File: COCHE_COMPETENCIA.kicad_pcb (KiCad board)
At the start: 2 copper layers, 90 x 65 mm, 25 parts, among them J1 BAT, J2 SENSORES, J3 M1, J4 M2, SW1 SW_Push, SW2 SW_Push, U1 L7805, U2 ESP32-DEVKIT-V1, U3 DRV8833, U4 DRV8833

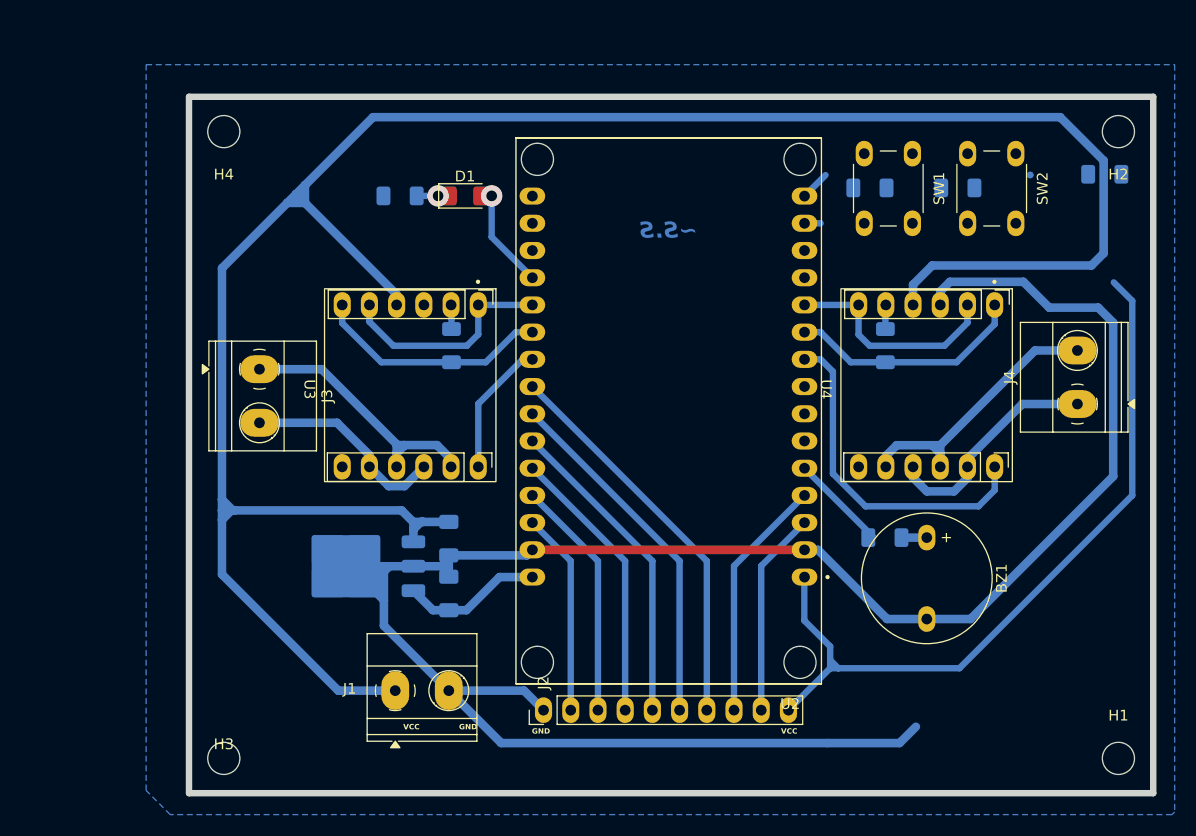
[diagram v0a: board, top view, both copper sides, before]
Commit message: V1 - MotorBoard 2025
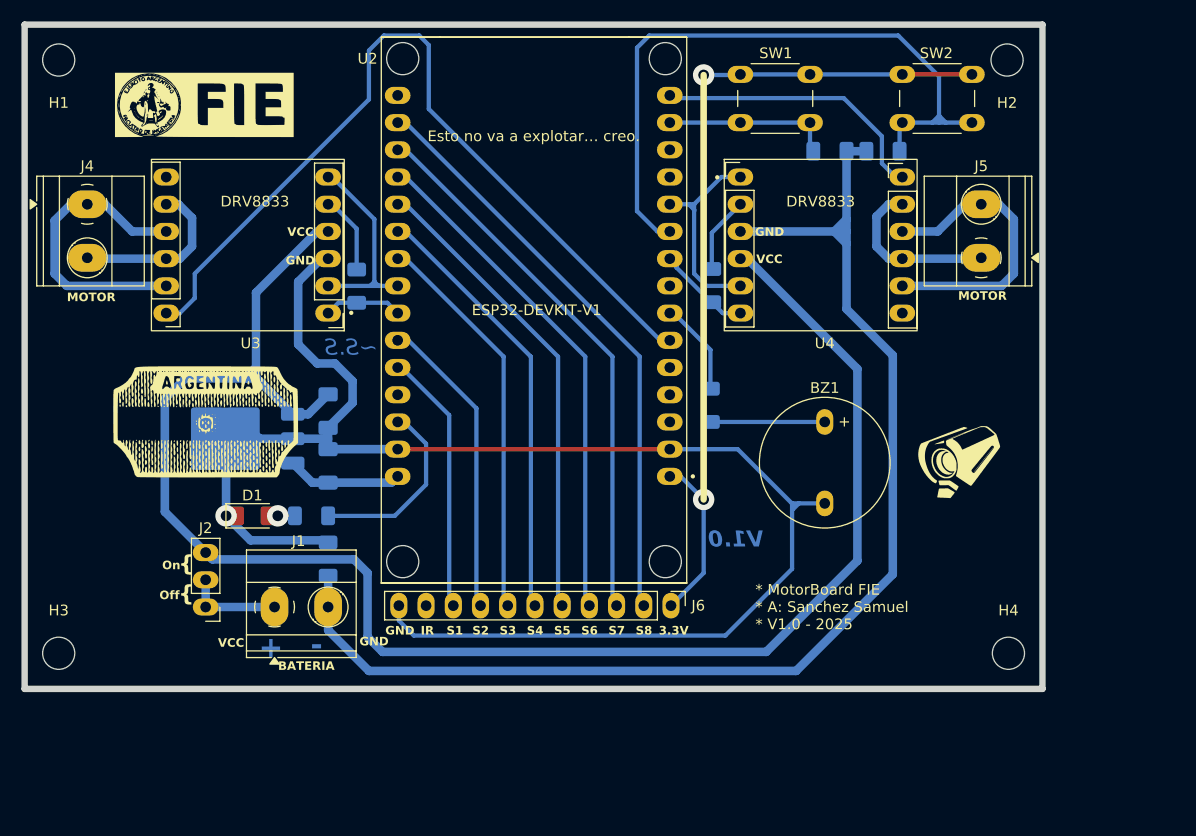
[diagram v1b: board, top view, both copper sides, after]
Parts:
- added G***: LOGO, LOGO, F.Cu at (114.6, 61.8)
- added G***: LOGO, LOGO, F.Cu at (184.8, 65.6)
- added G***: LOGO, LOGO, F.Cu at (114.4, 32.3)
- added J6: SENSORES, Connector_PinHeader_2.54mm:PinHeader_1x11_P2.54mm_Vertical, F.Cu at (158.0, 79.0)
- J2: value SENSORES -> SWITCH; footprint Connector_PinHeader_2.54mm:PinHeader_1x10_P2.54mm_Vertical -> Connector_PinHeader_2.54mm:PinHeader_1x03_P2.54mm_Vertical
- R1: value 10k -> 0
- R3: value 220 -> 10k
- R4: value 0 -> 220
- moved H1 118.5 mm to (100.8, 28.1), turned to 180 degrees
- moved H4 87.9 mm to (189.5, 83.4), turned to 0 degrees
- moved R1 61.3 mm to (126.0, 74.7), turned to -90 degrees
- moved R5 54.6 mm to (128.7, 49.2), turned to 90 degrees
- moved R3 45.3 mm to (177.8, 36.6)
- moved R7 42.7 mm to (161.7, 60.3), turned to -90 degrees
- moved D1 35.9 mm to (118.9, 70.6)
- moved J2 33.0 mm to (114.6, 79.1), turned to 180 degrees
- moved U3 24.0 mm to (118.1, 35.4), turned to 180 degrees
- moved J4 22.3 mm to (103.5, 41.5)
- moved R4 20.6 mm to (124.4, 70.6), turned to 180 degrees
- moved H3 18.3 mm to (100.8, 83.4)
- moved SW1 17.7 mm to (164.5, 29.4), turned to 0 degrees
- moved R6 17.1 mm to (161.8, 49.1)
- moved C1 16.4 mm to (126.0, 60.8)
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- renumbered J3 to J4, J4 to J5
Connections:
- net Net-(U1-OUT) renamed +5V
- D1 pad 1: Net-(D1-K) -> GND
- D1 pad 2: /LED_LARGADA -> Net-(D1-A)
- J1 pad 1: VCC -> Net-(J1-Pin_1)
- J2 pad 1: GND -> Net-(J1-Pin_1)
- J2 pad 2: /S1 -> Net-(J1-Pin_1)
- J2 pad 3: /S2 -> VCC
- R1 pad 1: /SW1 -> GND
- R2 pad 1: /SW2 -> /SW1
- R3 pad 1: Net-(D1-K) -> /SW2
- R4 pad 1: /IN_M1_B -> /LED_LARGADA
- R4 pad 2: Net-(U3-IN3) -> Net-(D1-A)
- R5 pad 1: /BUZZER -> /IN_M1_A
- R5 pad 2: Net-(BZ1-+) -> Net-(U3-IN2)
- R6 pad 1: /IN_M2_A -> /IN_M2_B
- R6 pad 2: Net-(U4-IN2) -> Net-(U4-IN3)
- R7 pad 1: +3.3V -> /BUZZER
- R7 pad 2: Net-(R7-Pad2) -> Net-(BZ1-+)
- SW1 pad 1: Net-(R7-Pad2) -> +3.3V
- SW2 pad 1: Net-(R7-Pad2) -> +3.3V
- U2 pad 10: /IN_M2_A -> /SW2
- U2 pad 11: /IN_M2_B -> /IN_M2_A
- U2 pad 14: /SW2 -> /SW1
- U2 pad 15: /SW1 -> /SLEEP_M2
- U2 pad 17: unconnected-(U2-VP-Pad17) -> /S8
- U2 pad 18: unconnected-(U2-VN-Pad18) -> /S7
- U2 pad 19: /LED_LARGADA -> /S6
- U2 pad 20: /IN_M1_A -> /S5
- U2 pad 21: /IN_M1_B -> /S4
- U2 pad 22: /SLEEP_M1 -> /S3
- U2 pad 23: /S6 -> /IN_M1_B
- U2 pad 24: /S5 -> /IN_M1_A
- U2 pad 25: /S4 -> /S2
- U2 pad 26: /S3 -> /S1
- U2 pad 27: /S2 -> unconnected-(U2-D12-Pad27)
- U2 pad 28: /S1 -> /LED_LARGADA
- U2 pad 3: /S8 -> unconnected-(U2-D15-Pad3)
- U2 pad 4: /S7 -> unconnected-(U2-D2-Pad4)
- U2 pad 5: /BUZZER -> unconnected-(U2-D4-Pad5)
- U2 pad 6: unconnected-(U2-RX2-Pad6) -> /SLEEP_M1
- U2 pad 7: unconnected-(U2-TX2-Pad7) -> /BUZZER
- U2 pad 9: /SLEEP_M2 -> /IN_M2_B
- U3 pad 2: Net-(U3-IN3) -> /IN_M1_B
- U3 pad 5: /IN_M1_A -> Net-(U3-IN2)
- U4 pad 2: /IN_M2_B -> Net-(U4-IN3)
- U4 pad 5: Net-(U4-IN2) -> /IN_M2_A
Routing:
- net GND: track 188.5 -> 269.8 mm, vias 0 -> 1
- net /SLEEP_M1: track 12.7 -> 77.0 mm
- net /SW2: track 1.56 -> 64.7 mm
- net VCC: track 213.9 -> 157.4 mm
- net /S8: track 19.2 -> 55.0 mm
- net /S7: track 22.8 -> 51.4 mm
- net /IN_M1_A: track 20.9 -> 7.29 mm
- net /SW1: track 2.77 -> 15.9 mm
- net /IN_M2_B: track 21.0 -> 8.89 mm
- net /S4: track 29.8 -> 40.7 mm
- net /S5: track 33.4 -> 44.3 mm
- net /S6: track 36.9 -> 47.9 mm
- net /S3: track 26.2 -> 37.1 mm
- net Net-(J1-Pin_1): track 0.00 -> 9.43 mm
- net +3.3V: track 71.6 -> 80.6 mm, vias 0 -> 2
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- removed copper zone on B.Cu, net GND
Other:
- board size 90 x 65 mm -> 95 x 62 mm
- board text added: "* MotorBoard FIE * A: Sanchez Samuel * V1.0 - 2025"
- board text added: "+"
- board text added: "-"
- board text added: "3.3V"
- board text added: "BATERIA"
- board text added: "DRV8833"
- board text added: "ESP32-DEVKIT-V1"
- board text added: "Esto no va a explotar… creo."
- board text added: "IR"
- board text added: "MOTOR"
- board text added: "Off"
- board text added: "On"
- board text added: "S1"
- board text added: "S2"
- board text added: "S3"
- board text added: "S4"
- board text added: "S5"
- board text added: "S6"
- board text added: "S7"
- board text added: "S8"
- board text added: "V1.0"
- board text added: "{"
